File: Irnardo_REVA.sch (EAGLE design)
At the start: 21 parts, among them J1 ICSP, U1 ATMEGA32U4-MU, U2 TSOP755, X1 16MHz

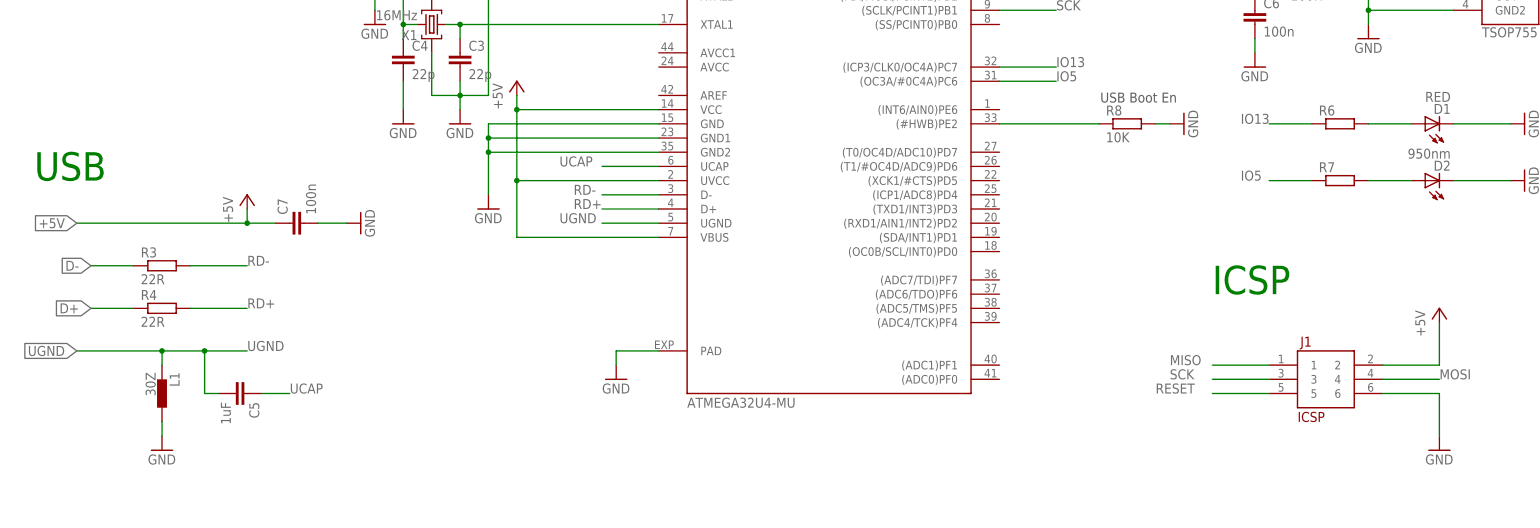
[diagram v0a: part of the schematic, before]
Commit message: First complete(ish) layout.
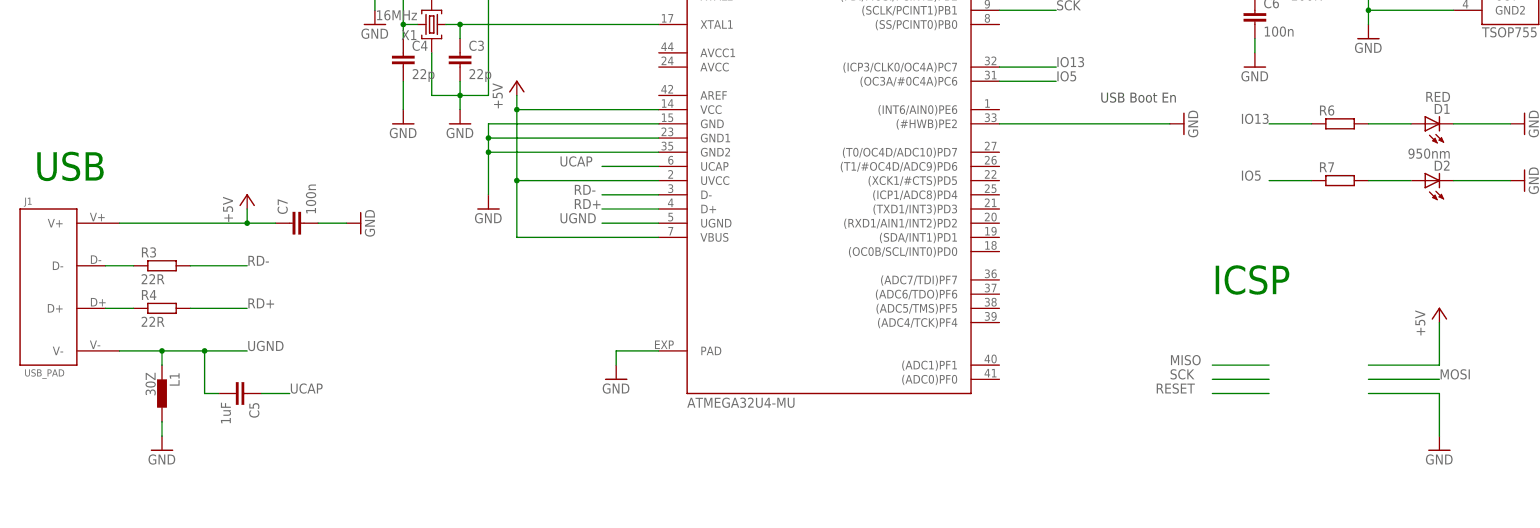
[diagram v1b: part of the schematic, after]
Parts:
- removed R8: 10K, resistor:R-EU_R0402
- J1: value ICSP -> USB_PAD; device 6X2005IN:6X2005IN -> USB_PAD:USB_PAD
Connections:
- removed net N$9: R8.1, U1.(#HWB)PE2
- net +5V: now also J1.V+; no longer J1.2
- net D+: now also J1.D+
- net D-: now also J1.D-
- net GND: now also U1.(#HWB)PE2; no longer J1.6, R8.2
- net MISO: no longer J1.1
- net MOSI: no longer J1.4
- net RESET: no longer J1.5
- net SCK: no longer J1.3
- net UGND: now also J1.V-
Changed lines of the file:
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@@
 <part name="D2" library="led" deviceset="LED" device="SML0603" value="950nm"/>
 <part name="GND10" library="supply1" deviceset="GND" device=""/>
-<part name="R8" library="resistor" deviceset="R-EU_" device="R0402" value="10K"/>
 <part name="GND11" library="supply1" deviceset="GND" device=""/>
 <part name="C7" library="resistor" deviceset="C-EU" device="C0402" value="100n"/>
@@
 <part name="P+5" library="supply1" deviceset="+5V" device=""/>
 <part name="GND13" library="supply1" deviceset="GND" device=""/>
-<part name="J1" library="6X2005IN" deviceset="6X2005IN" device="" value="ICSP"/>
+<part name="J1" library="USB_PAD" deviceset="USB_PAD" device=""/>
 </parts>
 <sheets>
@@
 <instance part="D2" gate="G$1" x="213.36" y="60.96" rot="R90"/>
 <instance part="GND10" gate="1" x="231.14" y="60.96" rot="R90"/>
-<instance part="R8" gate="G$1" x="160.02" y="71.12"/>
 <instance part="GND11" gate="1" x="170.18" y="71.12" rot="R90"/>
 <instance part="C7" gate="G$1" x="10.16" y="53.34" rot="R90"/>
@@
 <instance part="P+5" gate="1" x="215.9" y="38.1"/>
 <instance part="GND13" gate="1" x="215.9" y="12.7"/>
-<instance part="J1" gate="G$1" x="195.58" y="25.4"/>
+<instance part="J1" gate="G$1" x="-33.02" y="43.18"/>
 </instances>
 <busses>
@@
 <pinref part="P+2" gate="1" pin="+5V"/>
 <wire x1="2.54" y1="55.88" x2="2.54" y2="53.34" width="0.1524" layer="91"/>
-<wire x1="2.54" y1="53.34" x2="-27.94" y2="53.34" width="0.1524" layer="91"/>
-<label x="-27.94" y="53.34" size="1.778" layer="95" rot="R180" xref="yes"/>
+<wire x1="2.54" y1="53.34" x2="-20.32" y2="53.34" width="0.1524" layer="91"/>
 <pinref part="C7" gate="G$1" pin="1"/>
 <wire x1="2.54" y1="53.34" x2="7.62" y2="53.34" width="0.1524" layer="91"/>
 <junction x="2.54" y="53.34"/>
+<pinref part="J1" gate="G$1" pin="V+"/>
 </segment>
 <segment>
@@
 <segment>
 <pinref part="P+5" gate="1" pin="+5V"/>
-<wire x1="205.74" y1="27.94" x2="215.9" y2="27.94" width="0.1524" layer="91"/>
+<wire x1="203.2" y1="27.94" x2="215.9" y2="27.94" width="0.1524" layer="91"/>
 <wire x1="215.9" y1="27.94" x2="215.9" y2="35.56" width="0.1524" layer="91"/>
-<pinref part="J1" gate="G$1" pin="2"/>
 </segment>
 </net>
@@
 </segment>
 <segment>
-<pinref part="R8" gate="G$1" pin="2"/>
 <pinref part="GND11" gate="1" pin="GND"/>
-<wire x1="165.1" y1="71.12" x2="167.64" y2="71.12" width="0.1524" layer="91"/>
+<pinref part="U1" gate="G$1" pin="(#HWB)PE2"/>
+<wire x1="137.16" y1="71.12" x2="167.64" y2="71.12" width="0.1524" layer="91"/>
 </segment>
 <segment>
@@
 </segment>
 <segment>
-<wire x1="205.74" y1="22.86" x2="215.9" y2="22.86" width="0.1524" layer="91"/>
+<wire x1="203.2" y1="22.86" x2="215.9" y2="22.86" width="0.1524" layer="91"/>
 <pinref part="GND13" gate="1" pin="GND"/>
 <wire x1="215.9" y1="22.86" x2="215.9" y2="15.24" width="0.1524" layer="91"/>
-<pinref part="J1" gate="G$1" pin="6"/>
 </segment>
 </net>
@@
 <wire x1="185.42" y1="22.86" x2="175.26" y2="22.86" width="0.1524" layer="91"/>
 <label x="165.1" y="22.86" size="1.778" layer="95"/>
-<pinref part="J1" gate="G$1" pin="5"/>
 </segment>
 </net>
@@
 <pinref part="L1" gate="G$1" pin="1"/>
 <wire x1="-12.7" y1="27.94" x2="-12.7" y2="30.48" width="0.1524" layer="91"/>
-<wire x1="-12.7" y1="30.48" x2="-27.94" y2="30.48" width="0.1524" layer="91"/>
-<label x="-27.94" y="30.48" size="1.778" layer="95" rot="R180" xref="yes"/>
+<wire x1="-12.7" y1="30.48" x2="-20.32" y2="30.48" width="0.1524" layer="91"/>
 <label x="2.54" y="30.48" size="1.778" layer="95"/>
 <wire x1="-12.7" y1="30.48" x2="-5.08" y2="30.48" width="0.1524" layer="91"/>
@@
 <junction x="-12.7" y="30.48"/>
 <junction x="-5.08" y="30.48"/>
+<pinref part="J1" gate="G$1" pin="V-"/>
 </segment>
 </net>
@@
 <segment>
 <pinref part="R4" gate="G$1" pin="1"/>
-<wire x1="-17.78" y1="38.1" x2="-25.4" y2="38.1" width="0.1524" layer="91"/>
-<label x="-25.4" y="38.1" size="1.778" layer="95" rot="R180" xref="yes"/>
+<wire x1="-17.78" y1="38.1" x2="-22.86" y2="38.1" width="0.1524" layer="91"/>
+<pinref part="J1" gate="G$1" pin="D+"/>
 </segment>
 </net>
@@
 <segment>
 <pinref part="R3" gate="G$1" pin="1"/>
-<wire x1="-17.78" y1="45.72" x2="-25.4" y2="45.72" width="0.1524" layer="91"/>
-<label x="-25.4" y="45.72" size="1.778" layer="95" rot="R180" xref="yes"/>
+<wire x1="-17.78" y1="45.72" x2="-22.86" y2="45.72" width="0.1524" layer="91"/>
+<pinref part="J1" gate="G$1" pin="D-"/>
 </segment>
 </net>
@@
 </segment>
 </net>
-<net name="N$9" class="0">
-<segment>
-<pinref part="U1" gate="G$1" pin="(#HWB)PE2"/>
-<pinref part="R8" gate="G$1" pin="1"/>
-<wire x1="137.16" y1="71.12" x2="154.94" y2="71.12" width="0.1524" layer="91"/>
-</segment>
-</net>
 <net name="MISO" class="0">
 <segment>
@@
 <wire x1="185.42" y1="27.94" x2="175.26" y2="27.94" width="0.1524" layer="91"/>
 <label x="167.64" y="27.94" size="1.778" layer="95"/>
-<pinref part="J1" gate="G$1" pin="1"/>
 </segment>
 </net>
@@
 <wire x1="185.42" y1="25.4" x2="175.26" y2="25.4" width="0.1524" layer="91"/>
 <label x="167.64" y="25.4" size="1.778" layer="95"/>
-<pinref part="J1" gate="G$1" pin="3"/>
 </segment>
 </net>
@@
 </segment>
 <segment>
-<wire x1="205.74" y1="25.4" x2="215.9" y2="25.4" width="0.1524" layer="91"/>
+<wire x1="203.2" y1="25.4" x2="215.9" y2="25.4" width="0.1524" layer="91"/>
 <label x="215.9" y="25.4" size="1.778" layer="95"/>
-<pinref part="J1" gate="G$1" pin="4"/>
-</segment>
-</net>
+</segment>
+</net>
